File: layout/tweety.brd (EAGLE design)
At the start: 28 x 46 mm, 20 parts, among them IC2 MS563702BA03, P1 CR2450, U1 ATTINY88-MU

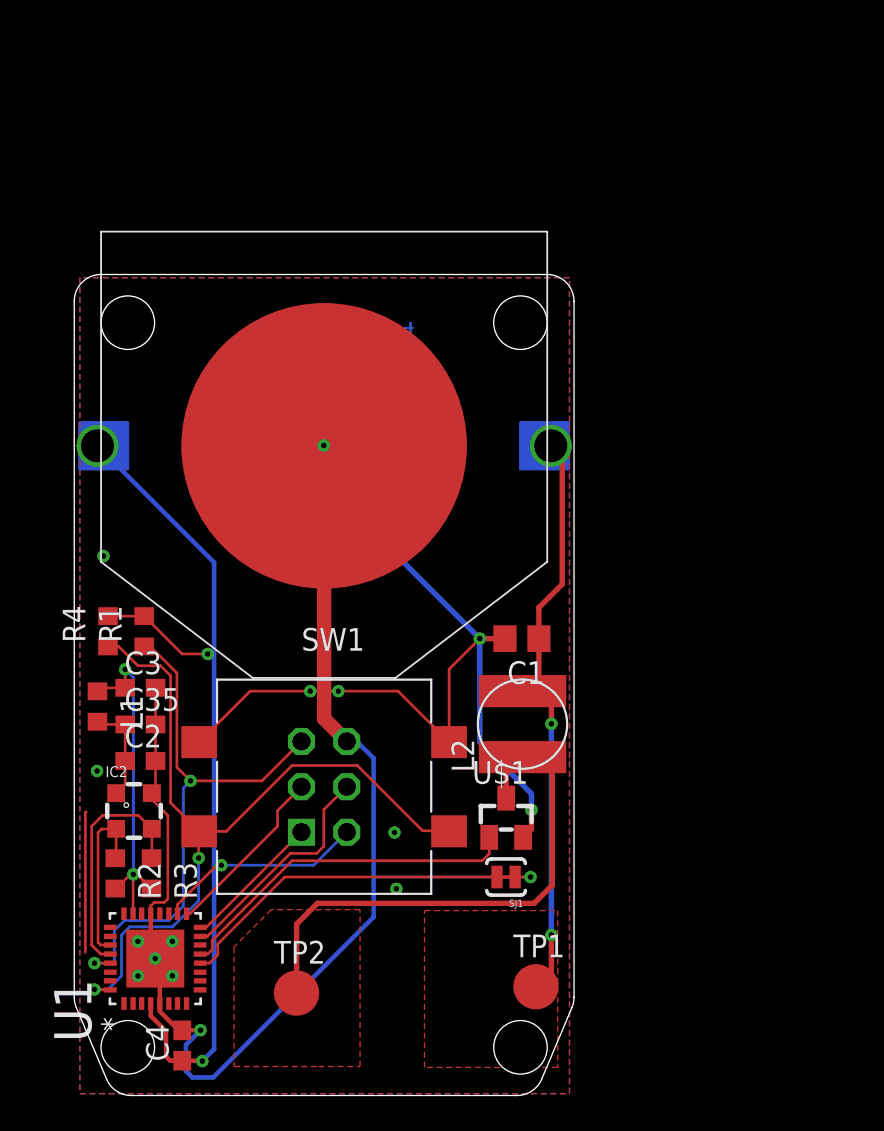
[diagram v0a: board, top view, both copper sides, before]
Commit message: v0.2
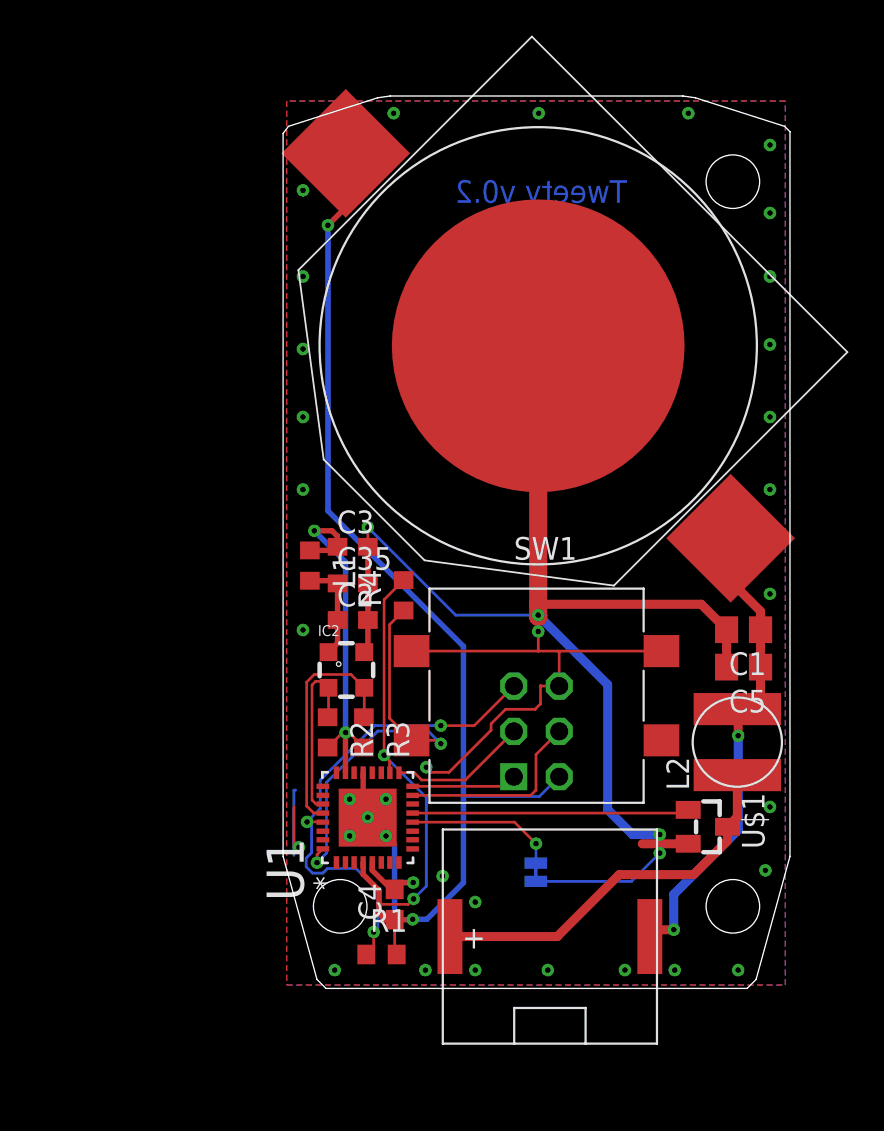
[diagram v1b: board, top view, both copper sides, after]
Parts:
- removed P1: CR2450, vario_spc:CR2450
- removed TP1, TP2: PTR1B2,54, testpad:B2,54
- added BAT1: KEYSTONE3008, vario_spc:KEYSTONE3008
- added C5: 10u, rcl-2:C0805
- added P2: PKLCS1212E2400, vario_spc:PKLCS1212
- L2: value sdr0503 10-15mH -> 4m7-15m
- moved R1 22.5 mm to (17.9, 7.80), turned to 0 degrees
- moved R4 16.7 mm to (19.2, 27.9)
- moved C3 14.3 mm to (16.3, 30.6)
- moved R3 14.3 mm to (16.9, 20.2)
- moved C2 14.3 mm to (16.3, 26.5)
- moved C35 14.3 mm to (16.3, 28.6)
- moved C4 14.3 mm to (18.7, 10.6)
- moved L1 14.3 mm to (13.9, 29.6)
- moved R2 14.3 mm to (14.9, 20.2)
- moved U1 14.3 mm to (17.1, 15.5)
- moved IC2 14.3 mm to (15.9, 23.7)
- moved SW1 12.9 mm to (26.6, 22.3)
- moved C1 12.4 mm to (38.2, 26.0)
- moved JP1 12.3 mm to (26.6, 20.3)
- moved L2 12.1 mm to (37.8, 19.7)
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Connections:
- new net N$5: U1.14
- net GND: now also BAT1.N, C5.2; no longer P1.N
- net N$2: no longer SW1.4
- net N$3: now also P2.P$+; no longer TP2.TP
- net VBAT: now also BAT1.P$3; no longer P1.P$1
- net VPP: now also BAT1.P$4, C5.1, P2.P$-; no longer P1.P$2, TP1.TP
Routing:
- net VBAT: track 61.8 -> 84.1 mm, vias 3 -> 4
- net N$2: track 44.7 -> 23.3 mm
- net GND: track 135.9 -> 122.9 mm, vias 16 -> 40
- net N$4: track 19.0 -> 8.52 mm, vias 0 -> 1
- net N$3: track 30.6 -> 21.7 mm
- net VPP: track 33.5 -> 27.7 mm
- net PIEZO: track 19.7 -> 15.5 mm
- net RESET: track 31.3 -> 27.9 mm, vias 2 -> 3
- net SCK: track 9.90 -> 7.73 mm
- net MOSI: track 12.9 -> 10.9 mm
- net MISO: track 7.89 -> 5.90 mm
- net VCC: track 19.3 -> 20.7 mm
- removed copper zone on layer 1, net N$3
- removed copper zone on layer 1, net VPP
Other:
- board size 28 x 46 mm -> 28.4 x 50 mm
- board text added: "Tweety v0.2"
- board text removed: "PCB thickness: 0.8mm"
- board text removed: "close gronund loop"
- board text removed: "height 6mm"
- board text removed: "tweety v0.1"
